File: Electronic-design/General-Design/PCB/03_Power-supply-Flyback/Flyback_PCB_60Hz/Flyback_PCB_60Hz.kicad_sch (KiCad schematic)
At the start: 56 parts, among them IC4 DPC817L-A-TR, IC5 UCC38C43DR, IC6 TL431ACLPR, J1 4300.0104, J5 TB002-500-02BE, Q1 BFR182E6327HTSA1, Q3 2N3906BU, Q4 Q_NMOS_GDS, T3 750811351

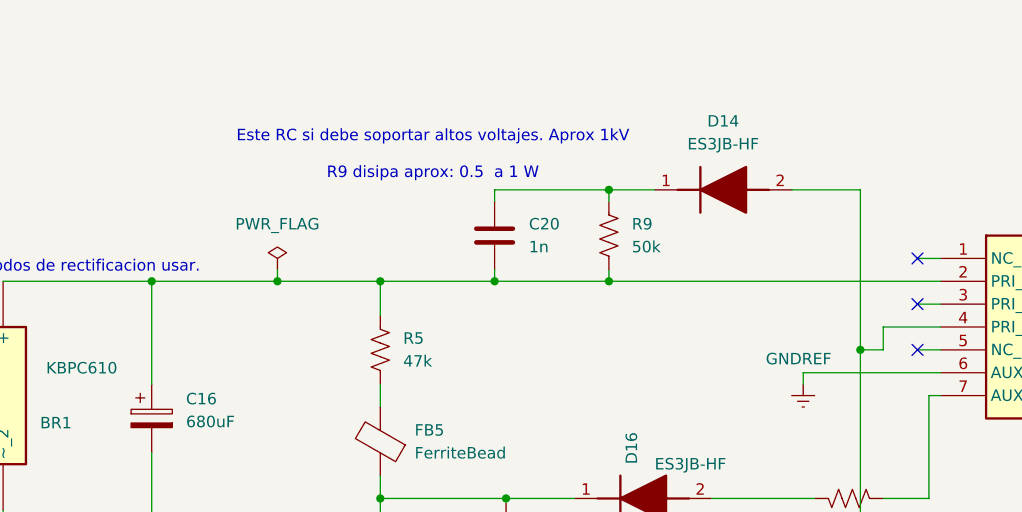
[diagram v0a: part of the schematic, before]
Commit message: Flyback-sch-correction2
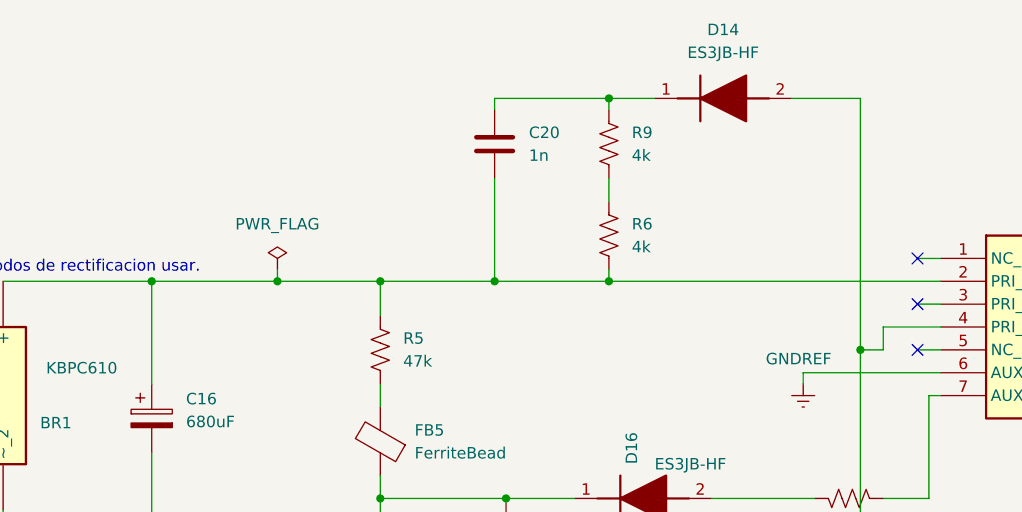
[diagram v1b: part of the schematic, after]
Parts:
- added R6: 4k, Resistor_THT:R_Axial_Power_L20.0mm_W6.4mm_P25.40mm, symbol Device:R_US
- R9: value 50k -> 4k; footprint Resistor_THT:R_Axial_Power_L50.0mm_W9.0mm_P60.96mm -> Resistor_THT:R_Axial_Power_L20.0mm_W6.4mm_P25.40mm
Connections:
- net at BR1.1 (+), C16.1, C20.2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: now also R6.2; no longer R9.2
- new net: R6.1, R9.2
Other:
- note removed: "Este RC si debe soportar altos voltajes. Aprox 1kV R9 disipa aprox: 0.5 a 1 W"
- moved on the sheet: C20, D14, R9
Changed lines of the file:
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@@
 	(generator_version "9.0")
 	(paper "A4")
-	(text "Este RC si debe soportar altos voltajes. Aprox 1kV\n\nR9 disipa aprox: 0.5  a 1 W"
-		(exclude_from_sim no)
-		(at 121.412 20.32 0)
-		(effects
-			(font
-				(size 1.27 1.27)
-			)
-		)
-	)
 	(text "Las resistencias 1206 soportan (R < 1k):\n	0.25W de disipacion. \n	200V max de nominal. \n	400\nV de trasientes cortos.\n\n	"
 		(exclude_from_sim no)
@@
 	)
 	(junction
-		(at 140.97 34.29)
-		(diameter 0)
-		(color 0 0 0 0)
-	)
-	(junction
 		(at 113.03 81.28)
 		(diameter 0)
@@
 	)
 	(junction
-		(at 140.97 24.13)
+		(at 140.97 13.97)
 		(diameter 0)
 		(color 0 0 0 0)
@@
 	)
 	(junction
+		(at 140.97 34.29)
+		(diameter 0)
+		(color 0 0 0 0)
+	)
+	(junction
 		(at 24.13 77.47)
 		(diameter 0)
@@
 	(wire
 		(pts
-			(xy 161.29 24.13) (xy 168.91 24.13)
+			(xy 161.29 13.97) (xy 168.91 13.97)
 		)
 		(stroke
@@
 	(wire
 		(pts
-			(xy 128.27 24.13) (xy 140.97 24.13)
+			(xy 128.27 13.97) (xy 140.97 13.97)
 		)
 		(stroke
@@
 	(wire
 		(pts
-			(xy 140.97 24.13) (xy 146.05 24.13)
+			(xy 140.97 13.97) (xy 146.05 13.97)
 		)
 		(stroke
@@
 	(wire
 		(pts
+			(xy 140.97 22.86) (xy 140.97 25.4)
+		)
+		(stroke
+			(width 0)
+			(type default)
+		)
+	)
+	(wire
+		(pts
 			(xy 255.27 31.75) (xy 255.27 33.02)
 		)
@@
 	(wire
 		(pts
-			(xy 140.97 34.29) (xy 140.97 33.02)
-		)
-		(stroke
-			(width 0)
-			(type default)
-		)
-	)
-	(wire
-		(pts
 			(xy 24.13 67.31) (xy 49.53 67.31)
 		)
@@
 	(wire
 		(pts
-			(xy 168.91 24.13) (xy 168.91 41.91)
+			(xy 168.91 13.97) (xy 168.91 41.91)
 		)
 		(stroke
@@
 	(wire
 		(pts
-			(xy 128.27 25.4) (xy 128.27 24.13)
+			(xy 128.27 15.24) (xy 128.27 13.97)
 		)
 		(stroke
@@
 	(wire
 		(pts
-			(xy 140.97 24.13) (xy 140.97 25.4)
+			(xy 140.97 13.97) (xy 140.97 15.24)
 		)
 		(stroke
@@
 	(wire
 		(pts
-			(xy 140.97 34.29) (xy 177.8 34.29)
+			(xy 128.27 34.29) (xy 140.97 34.29)
 		)
 		(stroke
@@
 	(wire
 		(pts
-			(xy 128.27 34.29) (xy 140.97 34.29)
-		)
-		(stroke
-			(width 0)
-			(type default)
-		)
-	)
-	(wire
-		(pts
 			(xy 36.83 90.17) (xy 36.83 91.44)
 		)
@@
 	(wire
 		(pts
-			(xy 128.27 34.29) (xy 128.27 33.02)
+			(xy 128.27 34.29) (xy 128.27 22.86)
 		)
 		(stroke
@@
 	(wire
 		(pts
+			(xy 140.97 33.02) (xy 140.97 34.29)
+		)
+		(stroke
+			(width 0)
+			(type default)
+		)
+	)
+	(wire
+		(pts
 			(xy 35.56 24.13) (xy 35.56 34.29)
 		)
@@
 	(wire
 		(pts
+			(xy 140.97 34.29) (xy 177.8 34.29)
+		)
+		(stroke
+			(width 0)
+			(type default)
+		)
+	)
+	(wire
+		(pts
 			(xy 135.89 83.82) (xy 135.89 85.09)
 		)
@@
 	(symbol
 		(lib_id "Device:R_US")
-		(at 140.97 29.21 0)
+		(at 140.97 19.05 0)
 		(unit 1)
 		(exclude_from_sim no)
@@
 		(fields_autoplaced yes)
 		(property "Reference" "R9"
-			(at 143.51 27.9399 0)
+			(at 143.51 17.7799 0)
 			(effects
 				(font
@@
 			)
 		)
-		(property "Value" "50k"
-			(at 143.51 30.4799 0)
+		(property "Value" "4k"
+			(at 143.51 20.3199 0)
 			(effects
 				(font
@@
 			)
 		)
-		(property "Footprint" "Resistor_THT:R_Axial_Power_L50.0mm_W9.0mm_P60.96mm"
-			(at 141.986 29.464 90)
+		(property "Footprint" "Resistor_THT:R_Axial_Power_L20.0mm_W6.4mm_P25.40mm"
+			(at 141.986 19.304 90)
 			(effects
 				(font
@@
 		)
 		(property "Datasheet" "~"
-			(at 140.97 29.21 0)
+			(at 140.97 19.05 0)
 			(effects
 				(font
@@
 		)
 		(property "Description" "Resistor, US symbol"
-			(at 140.97 29.21 0)
+			(at 140.97 19.05 0)
 			(effects
 				(font
@@
 	(symbol
 		(lib_id "F_1_ES3JB-HF:ES3JB-HF")
-		(at 146.05 24.13 0)
+		(at 146.05 13.97 0)
 		(unit 1)
 		(exclude_from_sim no)
@@
 		(fields_autoplaced yes)
 		(property "Reference" "D14"
-			(at 153.67 16.51 0)
+			(at 153.67 6.35 0)
 			(effects
 				(font
@@
 		)
 		(property "Value" "ES3JB-HF"
-			(at 153.67 19.05 0)
+			(at 153.67 8.89 0)
 			(effects
 				(font
@@
 		)
 		(property "Footprint" "Flyback:DIOM5235X244N"
-			(at 157.48 121.59 0)
+			(at 157.48 111.43 0)
 			(effects
 				(font
@@
 		)
 		(property "Datasheet" "https://www.comchiptech.com/admin/files/product/QW-JS017%20ES3AB-HF%20Thru.%20ES3JB-HF%20RevA.pdf"
-			(at 157.48 221.59 0)
+			(at 157.48 211.43 0)
 			(effects
 				(font
@@
 		)
 		(property "Description" "Rectifiers RECTIFIER SUPER FAST RECOVERY 600V 3A SMB"
-			(at 146.05 24.13 0)
+			(at 146.05 13.97 0)
 			(effects
 				(font
@@
 		)
 		(property "Height" "2.44"
-			(at 157.48 421.59 0)
+			(at 157.48 411.43 0)
 			(effects
 				(font
@@
 		)
 		(property "Mouser Part Number" "750-ES3JB-HF"
-			(at 157.48 521.59 0)
+			(at 157.48 511.43 0)
 			(effects
 				(font
@@
 		)
 		(property "Mouser Price/Stock" "https://www.mouser.co.uk/ProductDetail/Comchip-Technology/ES3JB-HF?qs=hd1VzrDQEGh59SJw6leQSQ%3D%3D"
-			(at 157.48 621.59 0)
+			(at 157.48 611.43 0)
 			(effects
 				(font
@@
 		)
 		(property "Manufacturer_Name" "Comchip Technology"
-			(at 157.48 721.59 0)
+			(at 157.48 711.43 0)
 			(effects
 				(font
@@
 		)
 		(property "Manufacturer_Part_Number" "ES3JB-HF"
-			(at 157.48 821.59 0)
+			(at 157.48 811.43 0)
 			(effects
 				(font
@@
 	(symbol
 		(lib_id "Device:C")
-		(at 128.27 29.21 0)
+		(at 128.27 19.05 0)
 		(unit 1)
 		(exclude_from_sim no)
@@
 		(fields_autoplaced yes)
 		(property "Reference" "C20"
-			(at 132.08 27.9399 0)
+			(at 132.08 17.7799 0)
 			(effects
 				(font
@@
 		)
 		(property "Value" "1n"
-			(at 132.08 30.4799 0)
+			(at 132.08 20.3199 0)
 			(effects
 				(font
@@
 		)
 		(property "Footprint" "Capacitor_THT:C_Disc_D7.5mm_W4.4mm_P5.00mm"
-			(at 129.2352 33.02 0)
+			(at 129.2352 22.86 0)
 			(effects
 				(font
@@
 		)
 		(property "Datasheet" "~"
-			(at 128.27 29.21 0)
+			(at 128.27 19.05 0)
 			(effects
 				(font
@@
 		)
 		(property "Description" "Unpolarized capacitor"
-			(at 128.27 29.21 0)
+			(at 128.27 19.05 0)
 			(effects
 				(font
@@
 					(unit 1)
 				)
+			)
+		)
+	)
+	(symbol
+		(lib_id "Device:R_US")
+		(at 140.97 29.21 0)
+		(unit 1)
+		(exclude_from_sim no)
+		(in_bom yes)
+		(on_board yes)
+		(dnp no)
+		(fields_autoplaced yes)
+		(property "Reference" "R6"
+			(at 143.51 27.9399 0)
+			(effects
+				(font
+					(size 1.27 1.27)
+				)
+				(justify left)
+			)
+		)
+		(property "Value" "4k"
+			(at 143.51 30.4799 0)
+			(effects
+				(font
+					(size 1.27 1.27)
+				)
+				(justify left)
+			)
+		)
+		(property "Footprint" "Resistor_THT:R_Axial_Power_L20.0mm_W6.4mm_P25.40mm"
+			(at 141.986 29.464 90)
+			(effects
+				(font
+					(size 1.27 1.27)
+				)
+				(hide yes)
+			)
+		)
+		(property "Datasheet" "~"
+			(at 140.97 29.21 0)
+			(effects
+				(font
+					(size 1.27 1.27)
+				)
+				(hide yes)
+			)
+		)
+		(property "Description" "Resistor, US symbol"
+			(at 140.97 29.21 0)
+			(effects
+				(font
+					(size 1.27 1.27)
+				)
+				(hide yes)
+			)
+		)
+		(pin "1"
+		)
+		(pin "2"
+		)
+		(instances
+			(project "Flyback_PCB_60Hz"
+				(path "/e667b3b5-58bf-48ce-ba71-7e90a3c6a4c9"
+					(reference "R6")
+					(unit 1)
+				)
